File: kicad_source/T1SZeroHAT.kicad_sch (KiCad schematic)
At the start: 48 parts, among them CN1 RASPI-IO, CN2 XY2500R-F-3.81-2P, CN3 SM02B-GHS-TB, CN4 SM02B-GHS-TB, SW1 SS-3235S-L3, U1 LAN8651, Y1 X1E0000210808

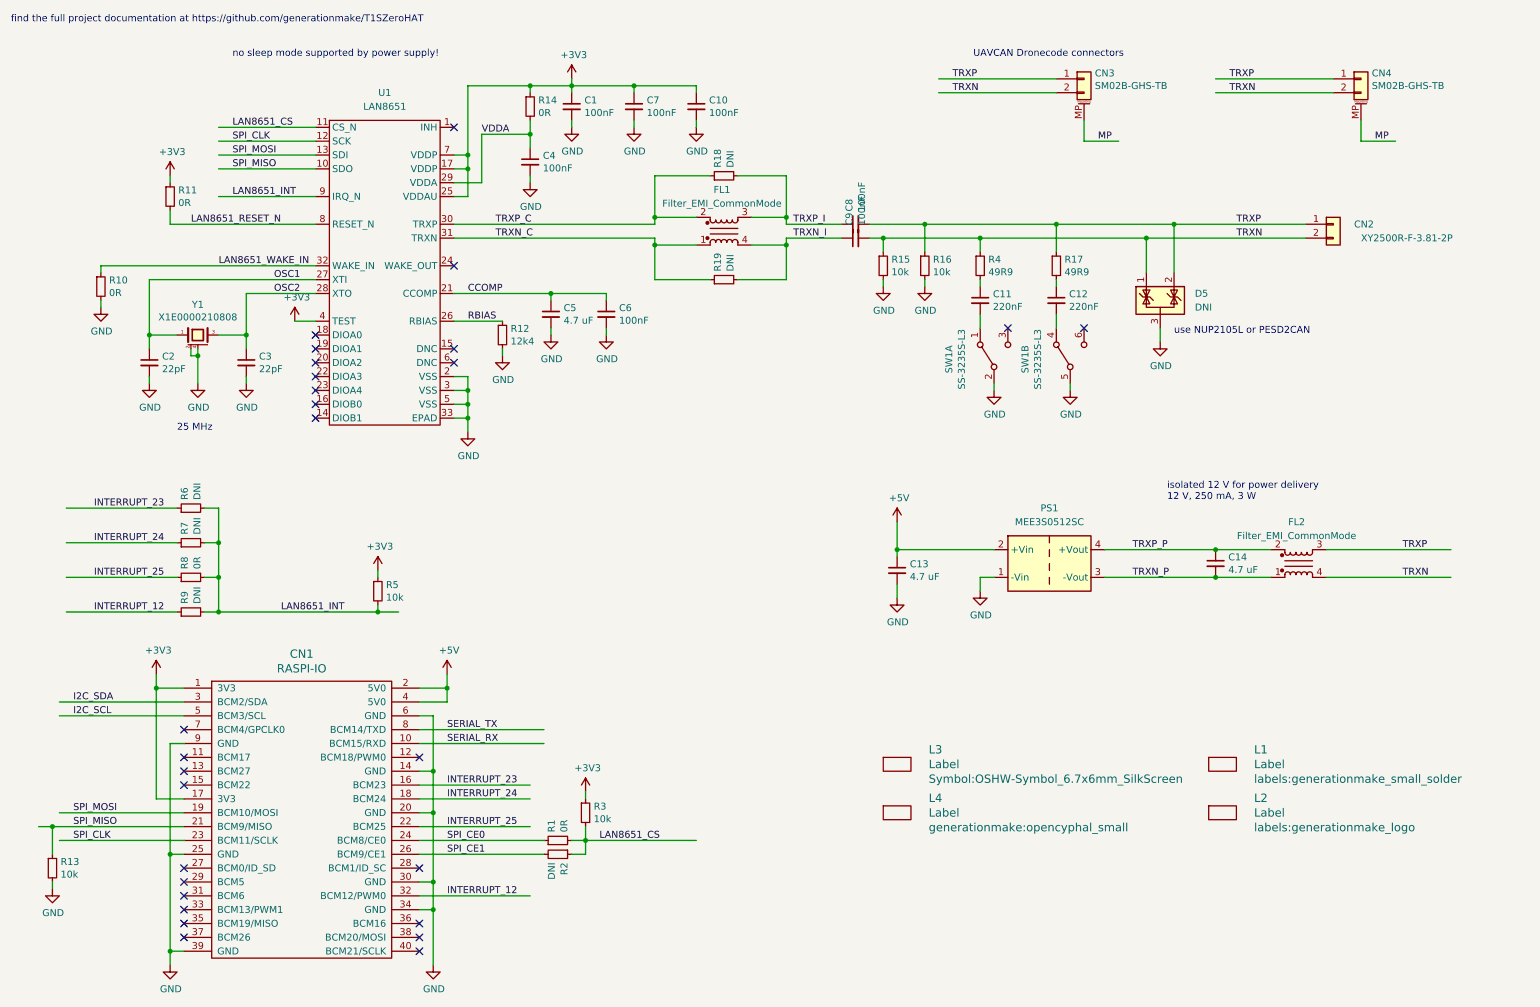
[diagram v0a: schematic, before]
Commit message: updated to kicad version 8
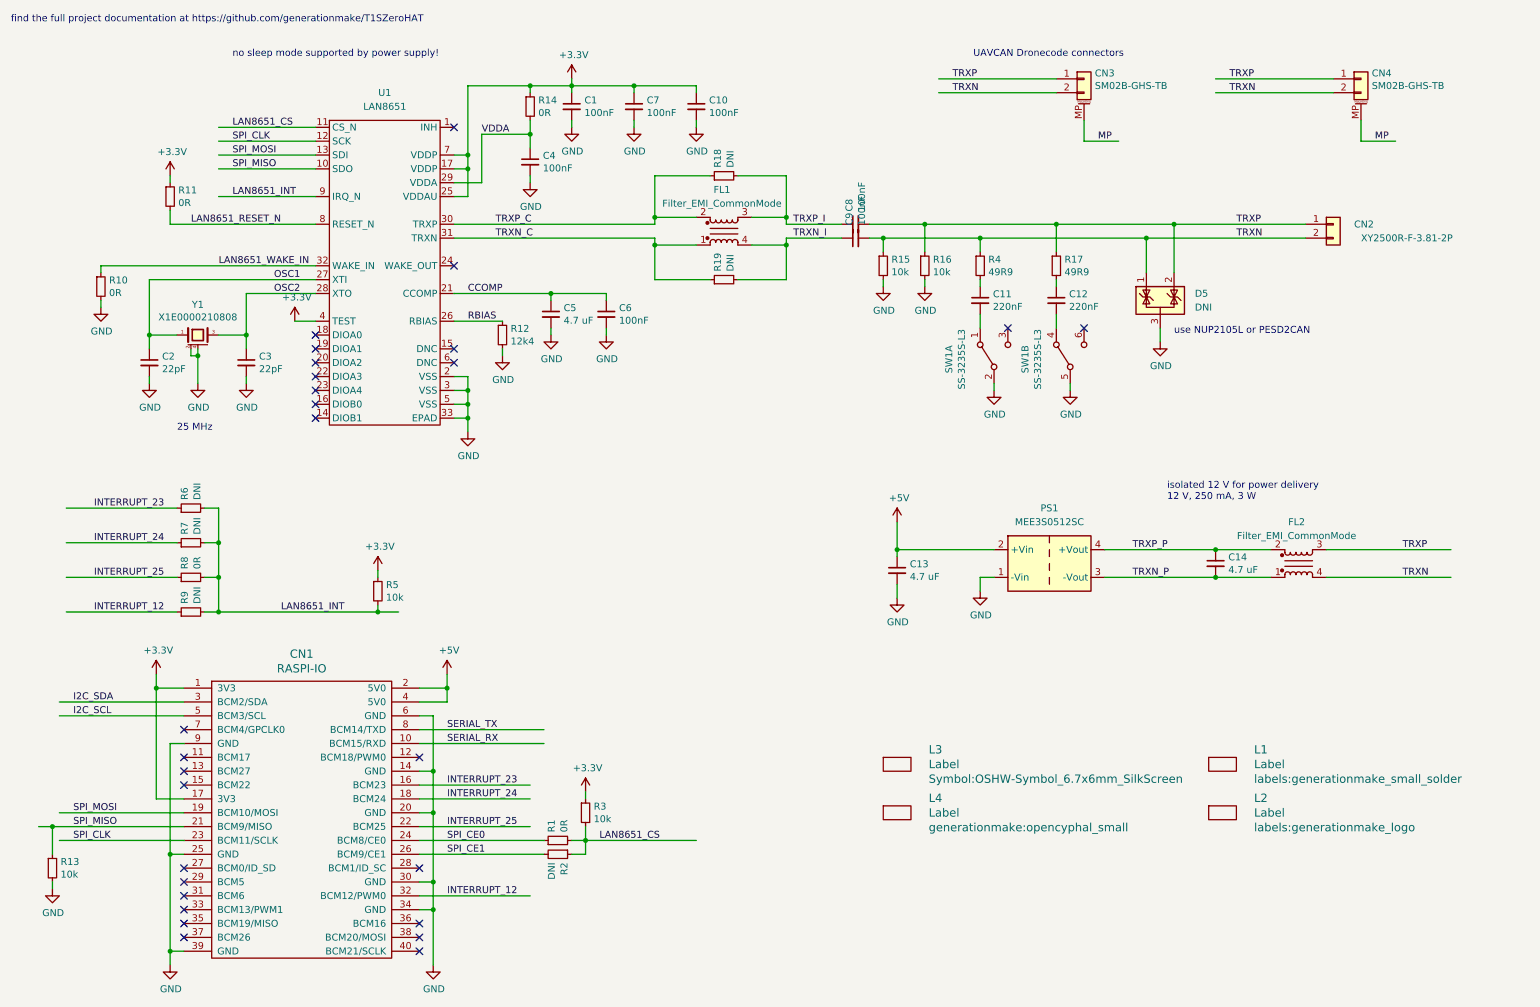
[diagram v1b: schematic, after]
